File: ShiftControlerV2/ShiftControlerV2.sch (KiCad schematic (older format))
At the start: 21 parts, among them Q1 BTN8982TA, Q2 BTN8982TA, U1 ControllerBoardV2

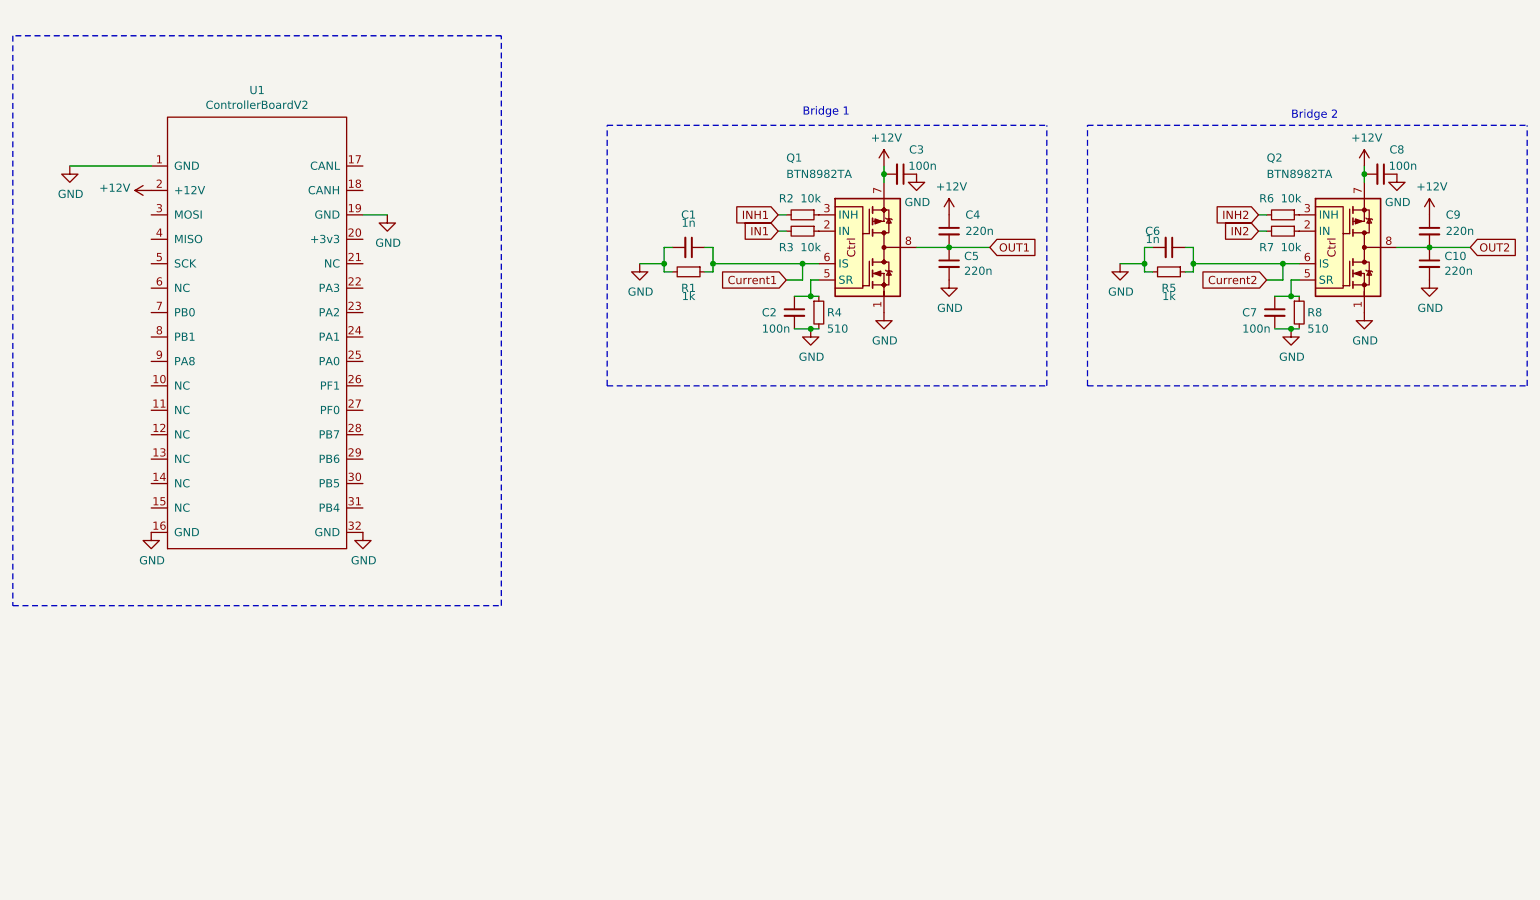
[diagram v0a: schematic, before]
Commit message: pcb detangled
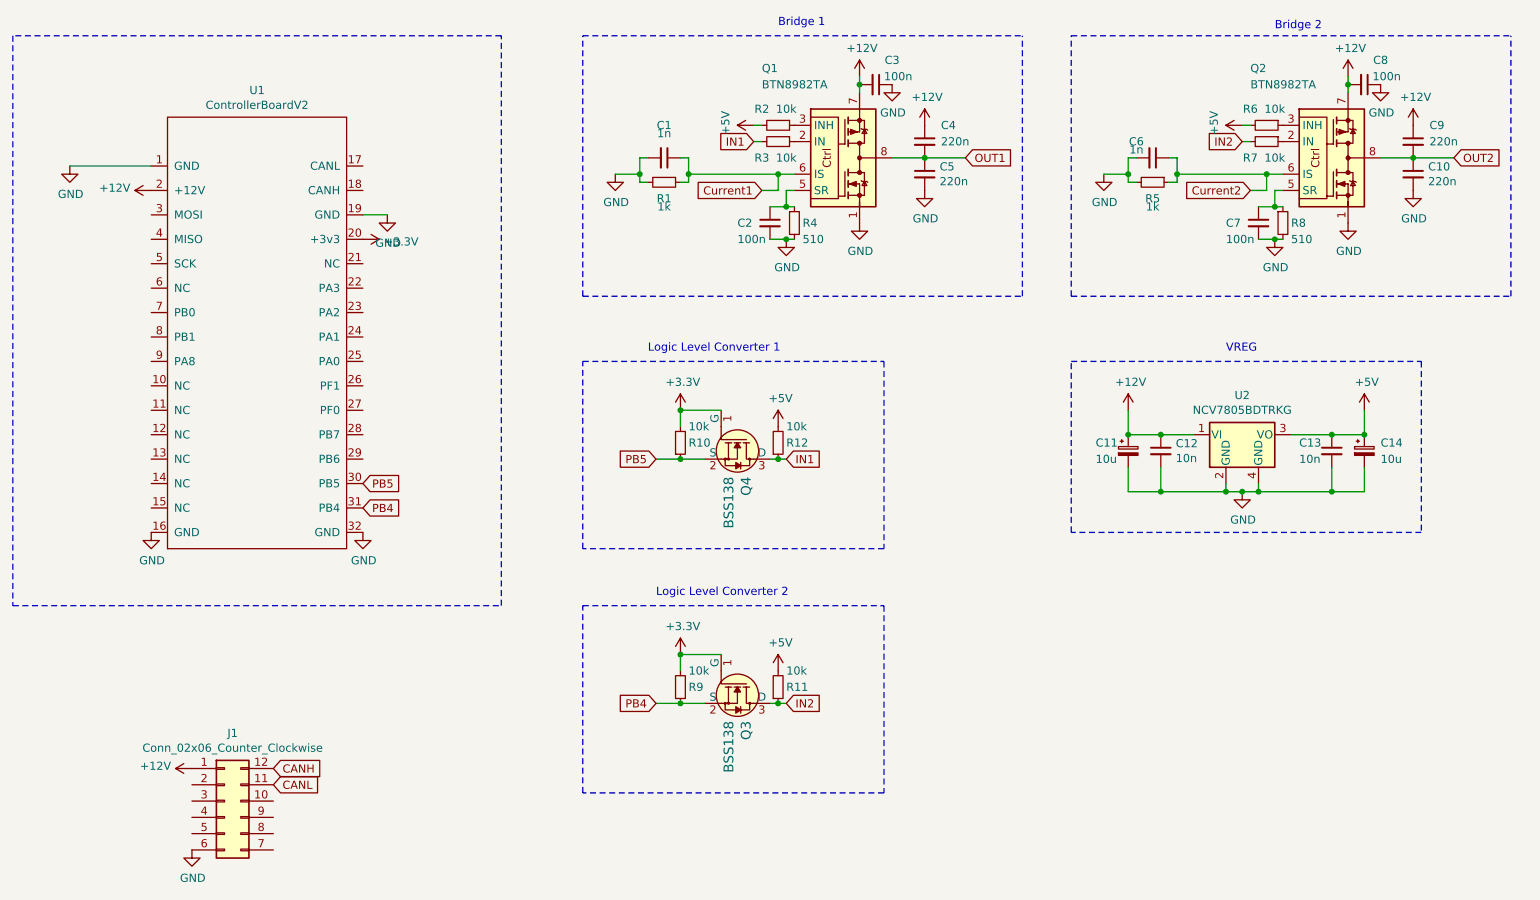
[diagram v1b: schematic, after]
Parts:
- added C11, C14: 10u, Capacitor_SMD:C_0201_0603Metric_Pad0.64x0.40mm_HandSolder, symbol Device:CP_Small
- added C12, C13: 10n, Capacitor_SMD:C_0201_0603Metric_Pad0.64x0.40mm_HandSolder, symbol Device:C_Small
- added J1: Conn_02x06_Counter_Clockwise, Lukas_Library:MX120G, symbol Connector_Generic:Conn_02x06_Counter_Clockwise
- added Q3, Q4: BSS138, digikey-footprints:SOT-23-3, symbol dk_Transistors-FETs-MOSFETs-Single:BSS138
- added R10, R11, R12, R9: 10k, Resistor_SMD:R_0201_0603Metric_Pad0.64x0.40mm_HandSolder, symbol Device:R_Small
- added U2: NCV7805BDTRKG, Package_TO_SOT_SMD:TO-252-3_TabPin4, symbol Lukas_Library:NCV7805BDTRKG
- C1, C10, C2, C3, C4, C5, C6, C7, C8, C9: footprint (none) -> Capacitor_SMD:C_0201_0603Metric_Pad0.64x0.40mm_HandSolder
- R1, R2, R3, R4, R5, R6, R7, R8: footprint (none) -> Resistor_SMD:R_0201_0603Metric_Pad0.64x0.40mm_HandSolder
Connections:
- net INH2 is gone; now on net +5V: R6.2
- net +12V: now also C11.1, C12.1, J1.1 (Pin_1), U2.1 (VI)
- net GND: now also C11.2, C12.2, C13.2, C14.2, J1.6 (Pin_6), U2.2 (GND), U2.4 (GND)
- net IN1: now also Q4.3 (D), R12.1
- net IN2: now also Q3.3 (D), R11.1
- net +3V3: now reaches U1.20 (+3v3)
- net +3V3: now also Q3.1 (G), Q4.1 (G), R10.2, R9.2
- net PB5: now reaches U1.30 (PB5)
- net PB5: now also Q4.2 (S), R10.1
- net PB4: now reaches U1.31 (PB4)
- net PB4: now also Q3.2 (S), R9.1
- net INH1 renamed +5V
- net +5V: now also C13.1, C14.1, R11.2, R12.2, U2.3 (VO)
- new net CANH: J1.12 (Pin_12)
- new net CANL: J1.11 (Pin_11)
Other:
- note added: "Logic Level Converter 1\n"
- note added: "Logic Level Converter 2"
- note added: "VREG"
- moved on the sheet: C1, C10, C2, C3, C4, C5, C6, C7, C8, C9, Q1, Q2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
